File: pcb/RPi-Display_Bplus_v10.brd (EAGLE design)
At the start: 85 x 56 mm, 42 parts, among them IC1 ADS7846, Q1 N-CHN, SW1 SW4S, U1 TS5204-3V3, X1 PASSER, X2 PASSER, X3 PASSER, X4 PASSER

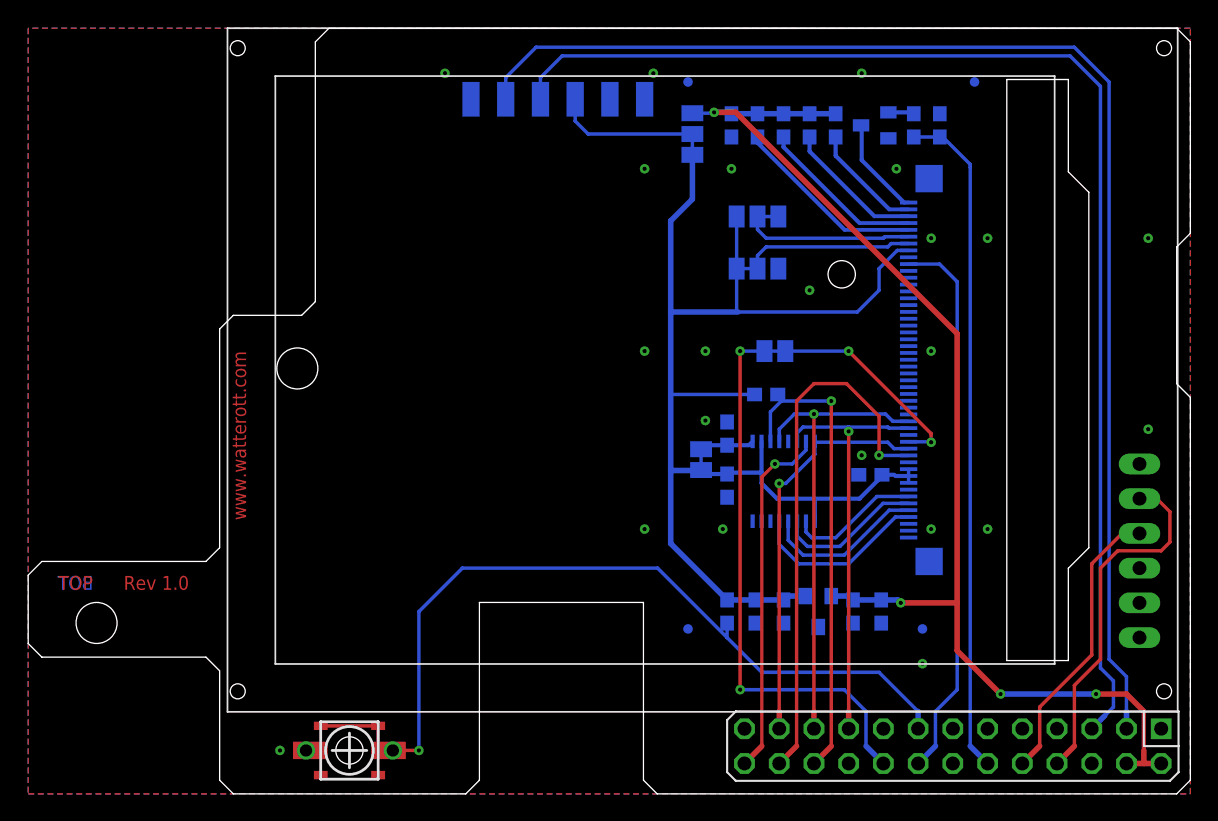
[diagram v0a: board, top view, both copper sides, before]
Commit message: updated layout and schematics
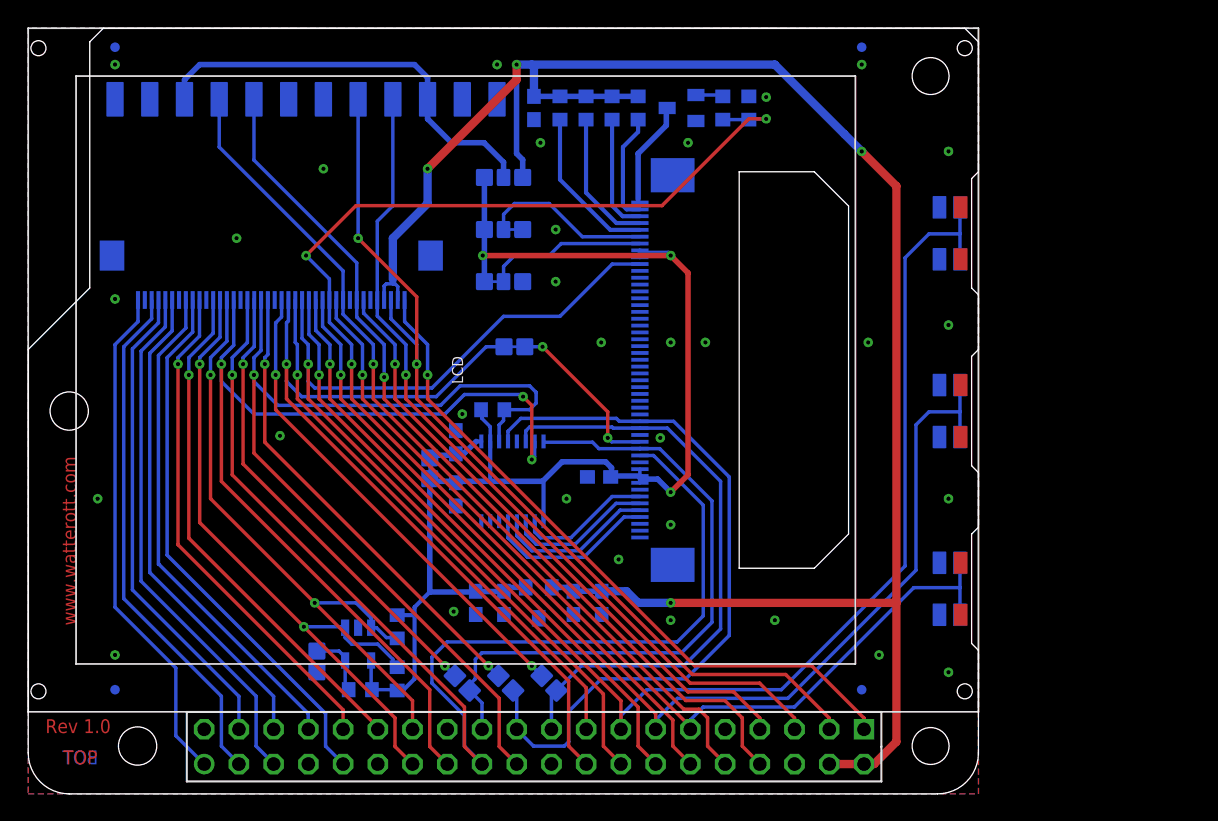
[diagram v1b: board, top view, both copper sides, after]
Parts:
- removed 1, 2, NC, NC.: WIREPADSMD1,27-254, wirepad:SMD1,27-2,54
- removed 3V3-5V: (no value), jumper:SJ_2
- removed FTDI: FTDI, Arduino:FTDI
- removed LCD1: MI0283QT9, Display:MI0283QT9
- added 5V-3V3: JUMPER3-NOCREAM, we-rcl:JUMPER3_NC
- added CTS, DTR, GND., NC1, NC2, RX, TX, VCC.: PAD-1.27-NC, we-rcl:PAD-1.27X2.54_NC
- added GPIO: FH12-40S-0.5SH, con-hirose:FH12-40S-0.5SH
- added IC2: 24LC-I/OT, we-chip:SOT23-5
- added LCD: MI0283QT-11, we-opto:MI0283QT11
- added LOGO2: WEEE_LOGO, we-symbol:WEEE
- added MISO, MOSI, SCK, WP: JUMPER2-NOCREAM, we-rcl:JUMPER2_NC
- added R10, R9: 3k9, rcl:R0603
- added SW2, SW3: SWITCH-PTS840P, we-switch:SW_PTS840P
- 3V3-VREF, IO24-RS: value (none) -> JUMPER2-NOCREAM; device jumper:SJ -> we-rcl:JUMPER2_NC
- C1, C4: value 1uF -> 2u
- C2, C3, C5, C6, C7, C8: value 100nF -> 100n
- GND, SCL, SDA, VCC: value WIREPADSMD1,27-254 -> PAD-1.27-NC; device wirepad:SMD1,27-2,54 -> we-rcl:PAD-1.27X2.54_NC
- IM0, IM1: value (none) -> JUMPER3-NOCREAM; device jumper:SJ_2 -> we-rcl:JUMPER3_NC
- R6: value 100k -> 47k
- R7: value 10k -> 47k
- R8: value 100k -> 3k9
- RPI: value (none) -> RPI; device RaspberryPi:RPI -> we-board:RPI_B+
- SW1: value SW4S -> SWITCH-PTS840P; device Switch-SMD:SW_SMD4 -> we-switch:SW_PTS840P
- moved U$1 61.6 mm to (68.9, 49.2), turned to 270 degrees
- moved SW1 45.5 mm to (67.4, 15.0), flipped to the bottom, turned to 270 degrees
- moved X1 42.1 mm to (6.35, 7.62)
- moved X2 42.0 mm to (6.35, 54.6)
- moved R8 34.1 mm to (27.0, 8.41), turned to 90 degrees
- moved RPI 30.6 mm to (37.0, 3.45)
- moved R7 22.6 mm to (34.0, 28.1), turned to 0 degrees
- moved LOGO1 22.5 mm to (18.1, 23.5), turned to 0 degrees
- moved C1 20.5 mm to (41.9, 14.0)
- moved C2 20.5 mm to (39.9, 14.0)
- moved C4 20.5 mm to (32.7, 14.0)
- moved C3 20.5 mm to (34.8, 14.0)
- moved U1 20.5 mm to (37.3, 14.0)
- moved 3V3-VREF 19.9 mm to (29.4, 23.8), turned to 180 degrees
- moved C5 19.9 mm to (31.3, 25.7)
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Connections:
- new net ID_SC: GPIO.13, IC2.1, R8.2, RPI.28
- new net ID_SD: GPIO.14, IC2.3, R9.2, RPI.27
- new net IO17: GPIO.30, RPI.11, SW1.3, SW1.4
- new net IO27: GPIO.28, RPI.13, SW2.3, SW2.4
- new net N$13: GPIO.24, RPI.17
- new net N$15: GPIO.12, RPI.29
- new net N$16: GPIO.10, RPI.31
- new net N$17: GPIO.8, RPI.33
- new net N$18: GPIO.6, RPI.35
- new net N$19: GPIO.4, RPI.37
- new net N$2: IC2.5, R10.2, WP.2
- new net N$25: GPIO.9, RPI.32
- new net N$27: GPIO.5, RPI.36
- new net N$28: GPIO.3, RPI.38
- new net N$29: GPIO.1, RPI.40
- new net N$4: GPIO.22, MOSI.1
- new net N$6: GPIO.20, MISO.1
- new net N$7: GPIO.18, SCK.1
- new net N$8: GPIO.40, RPI.1
- new net N$9: GPIO.34, RPI.7
- net +3V3: now also 5V-3V3.1, IC2.4, LCD.40, LCD.41, LCD.42, LCD.8, LCD.9, R10.1, R7.2, R8.1, R9.1; no longer 3V3-5V.1, LCD1.40, LCD1.41, LCD1.42, LCD1.8, R7.1, R8.2
- net +5V: now also 5V-3V3.3, GPIO.37, GPIO.39; no longer 3V3-5V.3
- net C1: now also LCD.1; no longer LCD1.1
- net GND: now also GND..1, GPIO.11, GPIO.16, GPIO.2, GPIO.21, GPIO.27, GPIO.32, GPIO.35, GPIO.7, IC2.2, LCD.11, LCD.12, LCD.13, LCD.14, LCD.15, LCD.16, LCD.17, LCD.18, LCD.19, LCD.20, LCD.21, LCD.22, LCD.23, LCD.24, LCD.25, LCD.26, LCD.27, LCD.28, LCD.29, LCD.30, LCD.31, LCD.32, LCD.35, LCD.43, LCD.48, LCD.49, LCD.50, RPI.14, RPI.20, RPI.30, RPI.34, RPI.39, RPI.9, SW1.2, SW2.1, SW2.2, SW3.1, SW3.2, WP.1; no longer 1.1, FTDI.1, LCD1.11, LCD1.12, LCD1.13, LCD1.14, LCD1.15, LCD1.16, LCD1.17, LCD1.18, LCD1.19, LCD1.20, LCD1.21, LCD1.22, LCD1.23, LCD1.24, LCD1.25, LCD1.26, LCD1.27, LCD1.28, LCD1.29, LCD1.30, LCD1.31, LCD1.32, LCD1.35, LCD1.43, LCD1.48, LCD1.49, LCD1.50, LCD1.9, SW1.4
- net IM0: now also LCD.6; no longer LCD1.6
- net IM1: now also LCD.7; no longer LCD1.7
- net IO18: now also GPIO.29
- net IO22: now also GPIO.26, SW3.3, SW3.4; no longer 2.1, R7.2, SW1.2, SW1.3
- net IO23: now also GPIO.25, LCD.10; no longer LCD1.10
- net IO24: now also GPIO.23
- net IO25: now also GPIO.19, R7.1; no longer R8.1
- net IO7: now also GPIO.15
- net IO8: now also GPIO.17, LCD.38; no longer LCD1.38
- net LED_A1: now also LCD.2; no longer LCD1.2
- net LED_A2: now also LCD.3; no longer LCD1.3
- net LED_A3: now also LCD.4; no longer LCD1.4
- net LED_A4: now also LCD.5; no longer LCD1.5
- net MISO: now also LCD.33, MISO.2; no longer LCD1.33
- net MOSI: now also LCD.34, MOSI.2; no longer LCD1.34
- net N$1: now also LCD.36; no longer LCD1.36
- net N$5: now also 5V-3V3.2, VCC..1; no longer 3V3-5V.2
- net RXD: now also GPIO.31, RX.1; no longer FTDI.4
- net SCK: now also LCD.37, SCK.2; no longer LCD1.37
- net SCL: now also GPIO.36
- net SDA: now also GPIO.38
- net TXD: now also GPIO.33, TX.1; no longer FTDI.5
- net X+: now also LCD.44; no longer LCD1.44
- net X-: now also LCD.46; no longer LCD1.46
- net Y+: now also LCD.45; no longer LCD1.45
- net Y-: now also LCD.47; no longer LCD1.47
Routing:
- net IO27: track 0.00 -> 83.8 mm, vias 0 -> 1
- net IO17: track 0.00 -> 70.4 mm, vias 0 -> 1
- net +5V: track 89.5 -> 144.8 mm
- net N$8: track 0.00 -> 50.3 mm, vias 0 -> 1
- net ID_SC: track 0.00 -> 49.6 mm, vias 0 -> 2
- net IO8: track 39.6 -> 86.6 mm
- net IO7: track 26.2 -> 72.4 mm, vias 1 -> 3
- net ID_SD: track 0.00 -> 45.6 mm, vias 0 -> 2
- net N$9: track 0.00 -> 45.4 mm, vias 0 -> 1
- net GND: track 0.00 -> 44.2 mm, vias 23 -> 32
- net RXD: track 21.1 -> 64.6 mm, vias 0 -> 1
- net IO18: track 49.3 -> 89.8 mm, vias 0 -> 3
- net N$13: track 0.00 -> 40.2 mm, vias 0 -> 1
- net N$25: track 0.00 -> 40.0 mm
- net TXD: track 26.3 -> 65.6 mm, vias 0 -> 1
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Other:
- board size 85 x 56 mm -> 69.5 x 56 mm
- board text added: "2.4mm PCB, Silkscreen: 22 bPlace + 26 bNames"
- board text added: "40"
- board text added: "8-Bit SPI"
- board text added: "I2C"
- board text added: "ID EEPROM"
- board text added: "Serial"
- board text removed: "2.0mm PCB, Silkscreen: 22 bPlace + 26 bNames"
